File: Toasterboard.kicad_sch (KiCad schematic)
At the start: 25 parts, among them J1 Power, J2 LEDs, J3 Switches, SW1 SW_SPDT, SW2 SW_SPDT, SW3 SW_SPDT, SW4 SW_SPDT, U1 LM341T-05_TO220, U2 NE555P, U3 74LS14

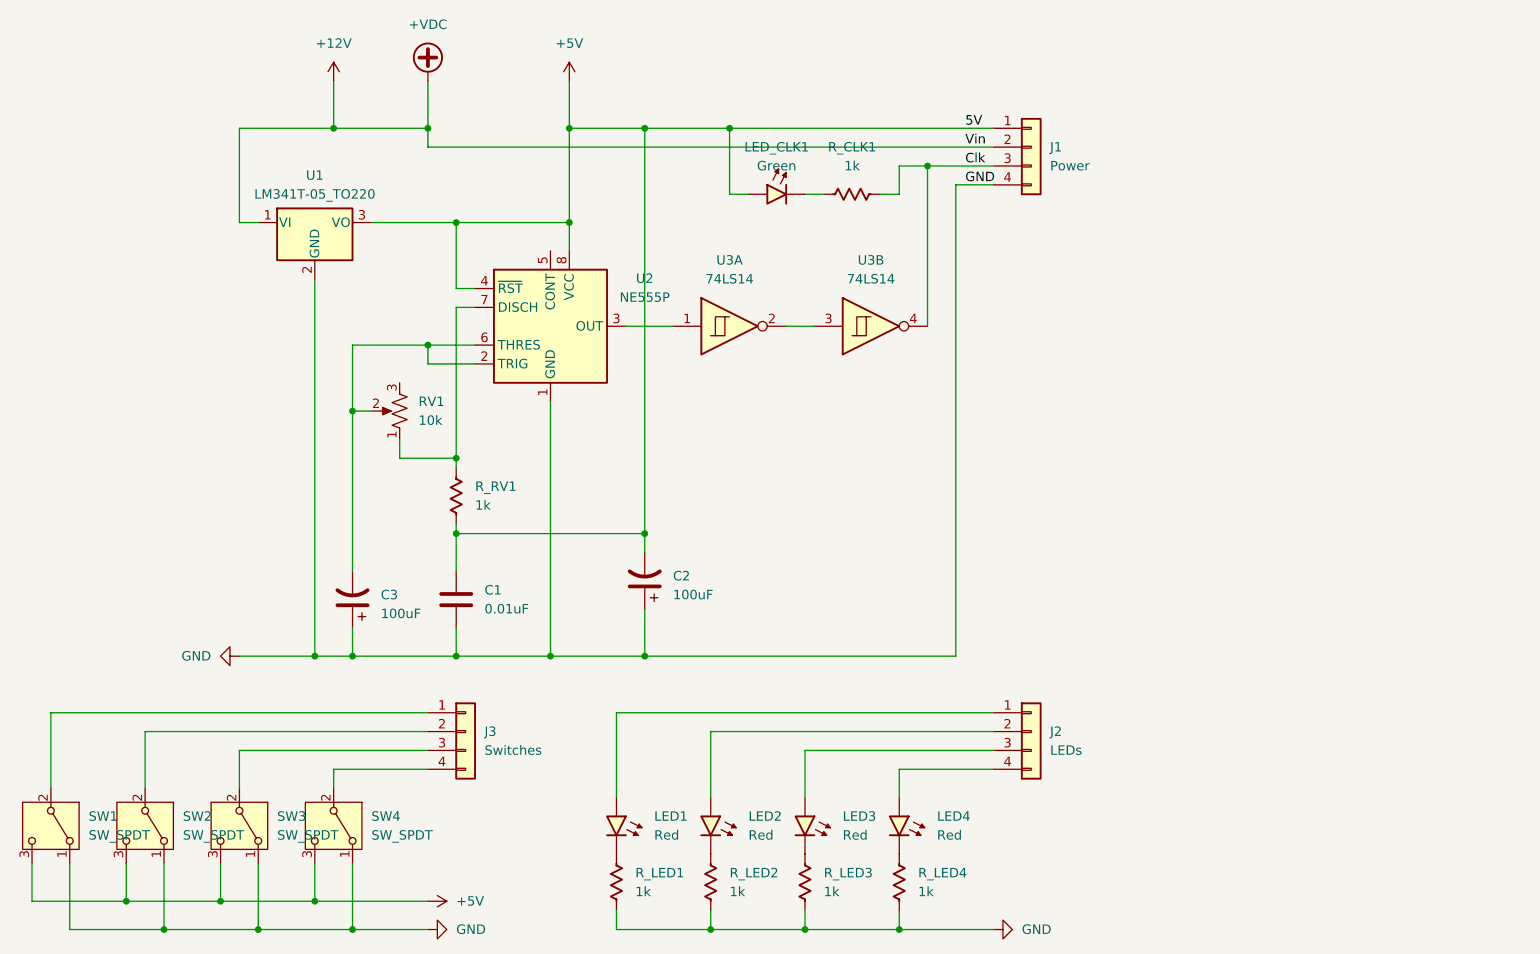
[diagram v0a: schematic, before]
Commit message: feat: finish routing
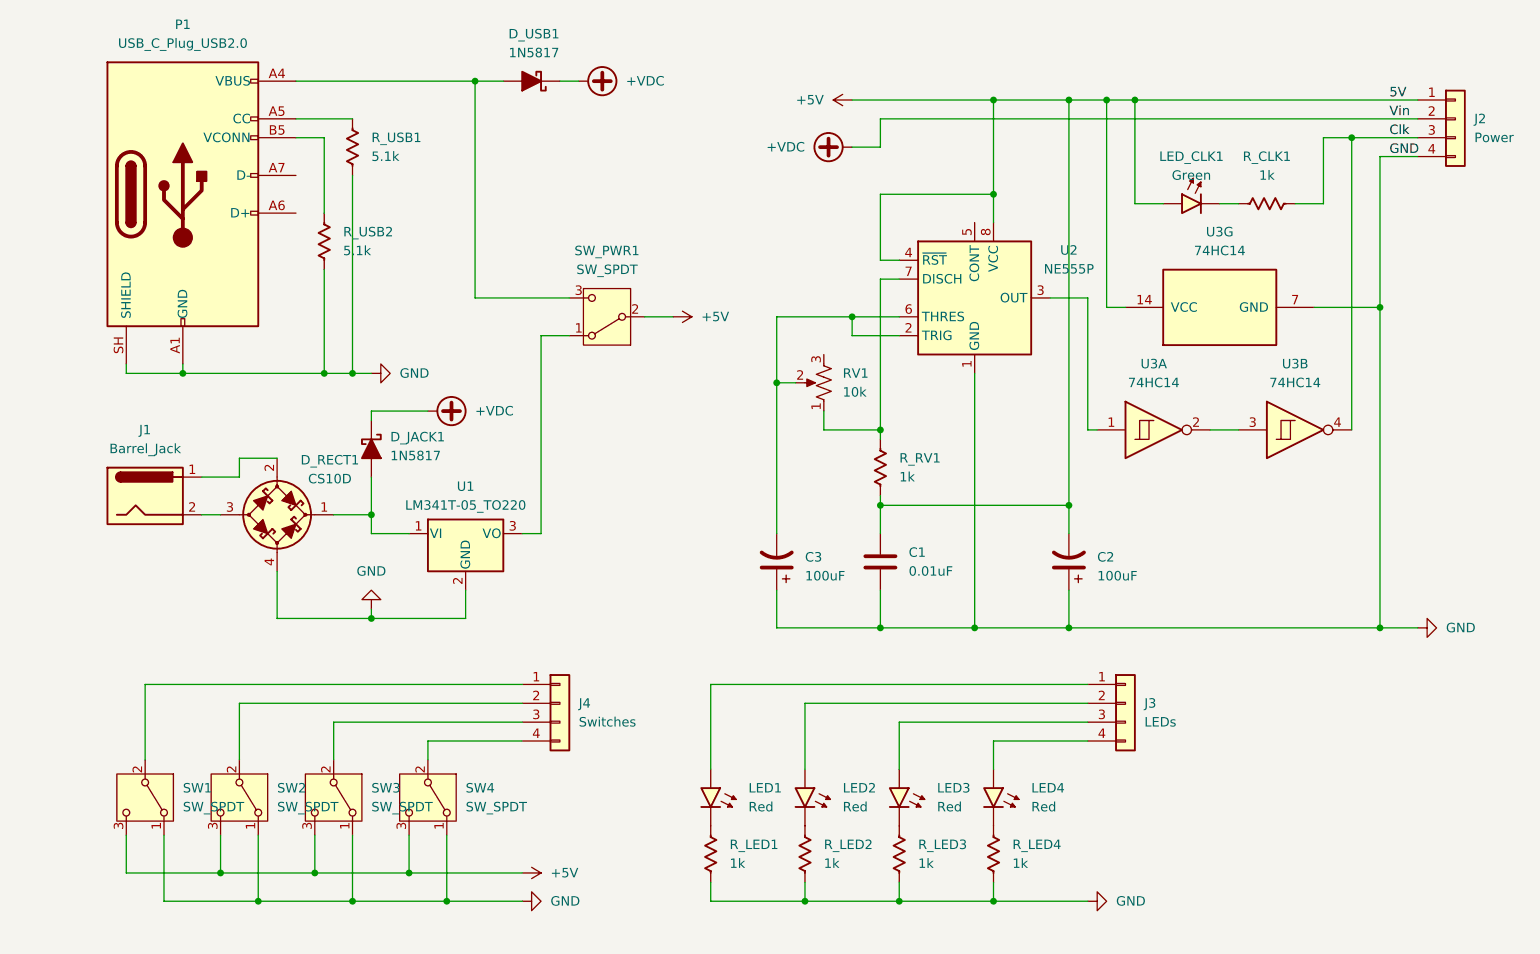
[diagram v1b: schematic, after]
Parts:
- added D_JACK1, D_USB1: 1N5817, Diode_THT:D_DO-41_SOD81_P2.54mm_Vertical_CathodeUp, symbol PCM_Diode_Schottky_AKL:1N5817
- added D_RECT1: CS10D, PCM_Diode_THT_AKL:Diode_Bridge_DIP-4_W7.62mm_P5.08mm, symbol PCM_Diode_Bridge_AKL:CS10D
- added J1: Barrel_Jack, Connector_BarrelJack:BarrelJack_GCT_DCJ200-10-A_Horizontal, symbol Connector:Barrel_Jack
- added P1: USB_C_Plug_USB2.0, Connector_USB:USB_C_Receptacle_GCT_USB4135-GF-A_6P_TopMnt_Horizontal, symbol Connector:USB_C_Plug_USB2.0
- added R_USB1, R_USB2: 5.1k, PCM_Resistor_THT_US_AKL:R_Axial_DIN0207_L6.3mm_D2.5mm_P2.54mm_Vertical, symbol PCM_Resistor_US_AKL:R_DIN0207_P5.08mm
- added SW_PWR1: SW_SPDT, Button_Switch_THT:SW_Slide_SPDT_Straight_CK_OS102011MS2Q, symbol Switch:SW_SPDT
- added unit 7 of U3
- R_CLK1, R_LED1, R_LED2, R_LED3, R_LED4: footprint PCM_Resistor_THT_US_AKL:R_Axial_DIN0207_L6.3mm_D2.5mm_P5.08mm_Vertical -> PCM_Resistor_THT_US_AKL:R_Axial_DIN0207_L6.3mm_D2.5mm_P2.54mm_Vertical
- U3: value 74LS14 -> 74HC14; symbol 74xx:74LS14 -> 74xx:74HC14
- renumbered J1 to J2, J2 to J3, J3 to J4
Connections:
- net +5V: now also SW_PWR1.2 (B), U3.14 (VCC); no longer U1.3 (VO)
- net GND: now also D_RECT1.4 (2), P1.A1 (GND), P1.A12 (GND), P1.B1 (GND), P1.B12 (GND), P1.SH (SHIELD), R_USB1.2, R_USB2.2, U3.7 (GND)
- net +12V: no longer names the net of U1.1 (VI)
- net +12V: now also D_JACK1.2 (A), D_RECT1.1 (+); no longer J2.2 (Pin_2)
- new net: D_RECT1.2 (1), J1.1
- new net: D_RECT1.3 (-), J1.2
- new net: P1.A5 (CC), R_USB1.1
- new net: D_USB1.2 (A), P1.A4 (VBUS), P1.A9 (VBUS), P1.B4 (VBUS), P1.B9 (VBUS), SW_PWR1.3 (C)
- new net: P1.B5 (VCONN), R_USB2.1
- new net: SW_PWR1.1 (A), U1.3 (VO)
- new net +VDC: D_JACK1.1 (K), D_USB1.1 (K), J2.2 (Pin_2)
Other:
- moved on the sheet: C1, C2, C3, J2, J3, J4, LED1, LED2, LED3, LED4, LED_CLK1, RV1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
